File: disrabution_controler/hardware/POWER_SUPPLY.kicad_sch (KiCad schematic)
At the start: 17 parts, among them Q18 NMOS, Q19 NMOS, U4 AP62150WU

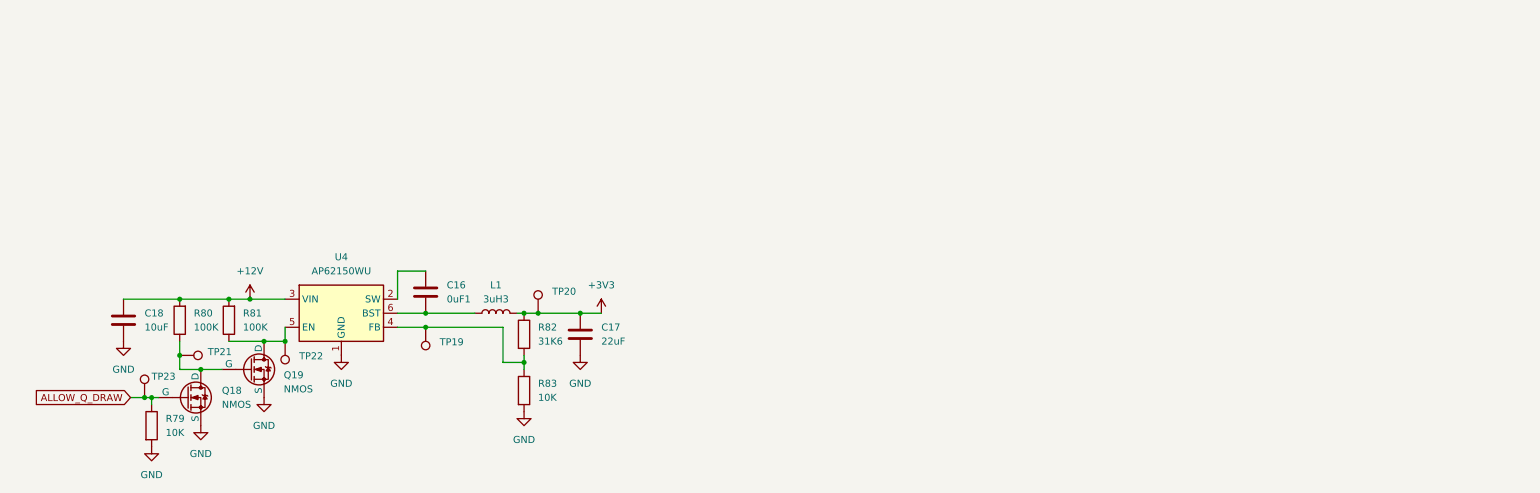
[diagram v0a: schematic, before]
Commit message: more hardware work
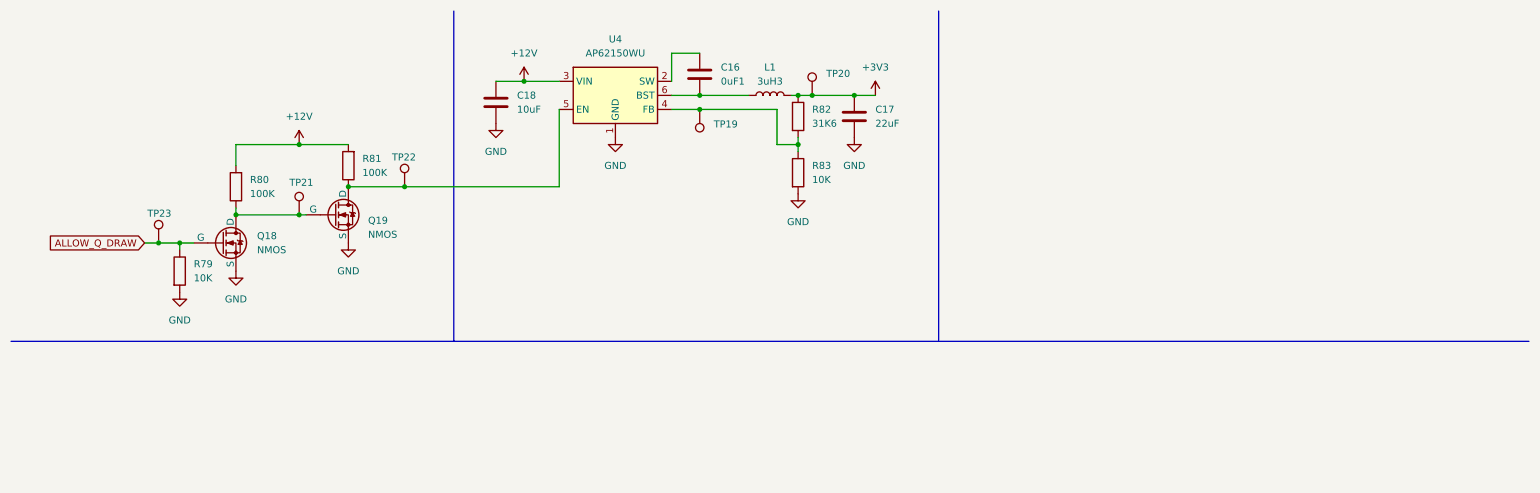
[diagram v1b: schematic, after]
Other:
- moved on the sheet: C16, C17, C18, L1, Q18, Q19, R79, R80, R81, R82, R83, TP19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
